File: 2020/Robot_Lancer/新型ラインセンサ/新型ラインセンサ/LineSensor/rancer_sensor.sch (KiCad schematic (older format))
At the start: 31 parts, among them P1 XH_08, U1 S7136, U2 TPR-105F, U3 TPR-105F, U4 S7136, U5 S7136

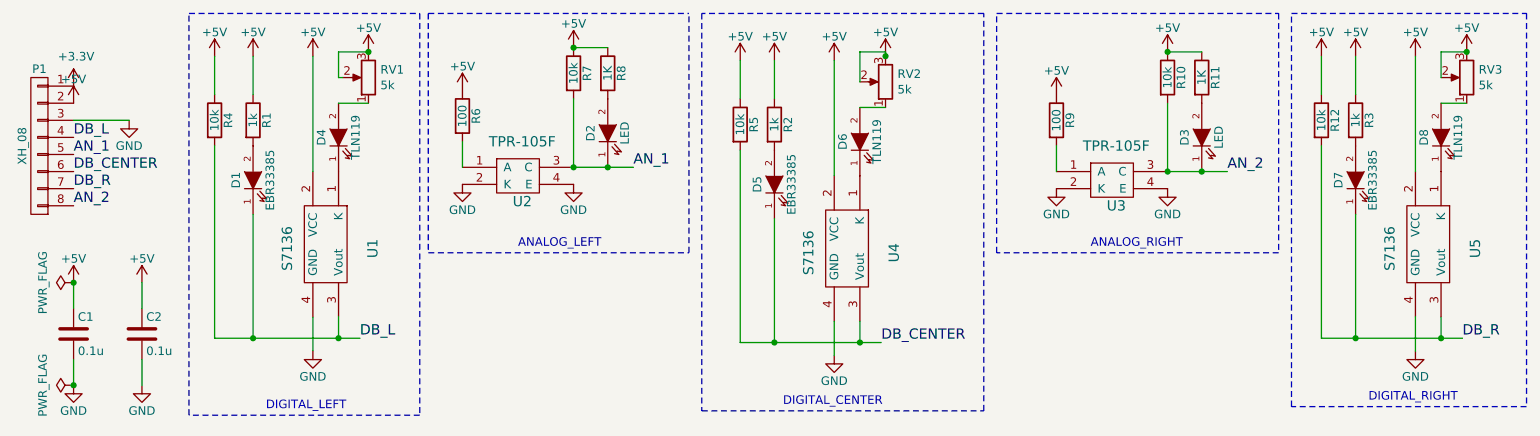
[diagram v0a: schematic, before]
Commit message: 小谷ランサー基板
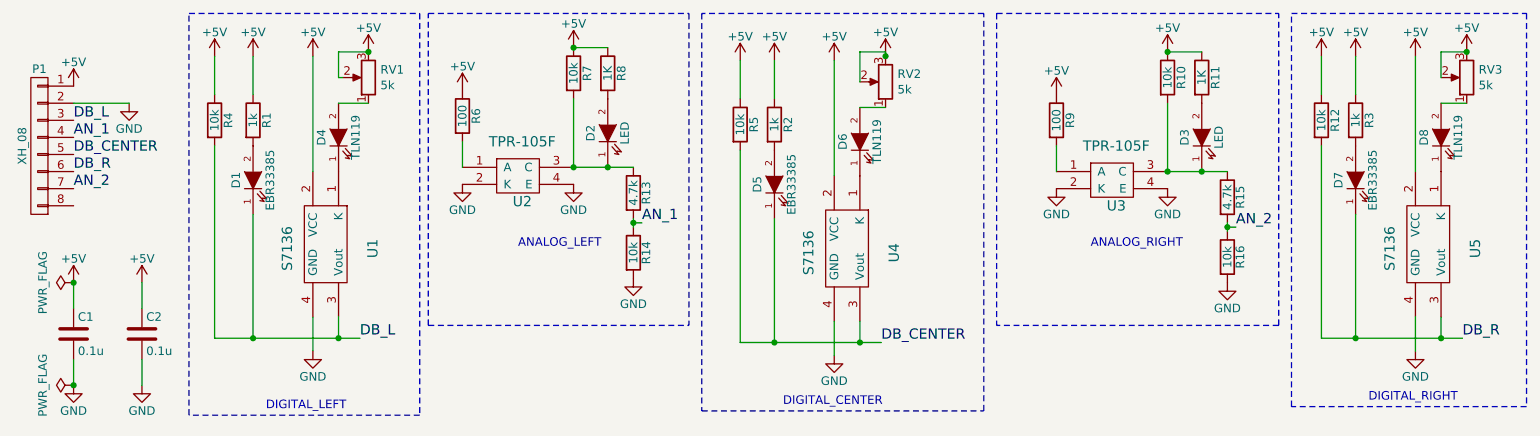
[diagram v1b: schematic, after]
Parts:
- added R13, R15: 4.7k, Mizz_lib:1608_WP, symbol Device:R
- added R14, R16: 10k, Mizz_lib:1608_WP, symbol Device:R
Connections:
- net +3V3 is gone; now on net +5V: P1.1 (P1)
- net +5V: no longer P1.2 (P2)
- net AN_1: now also P1.4 (P4), R13.2, R14.1; no longer D2.1 (K), P1.5 (P5), R7.2, U2.3 (C)
- net AN_2: now also P1.7 (P7), R15.2, R16.1; no longer D3.1 (K), P1.8 (P8), R10.2, U3.3 (C)
- net DB_CENTER: now also P1.5 (P5); no longer P1.6 (P6)
- net DB_L: now also P1.3 (P3); no longer P1.4 (P4)
- net DB_R: now also P1.6 (P6); no longer P1.7 (P7)
- net GND: now also P1.2 (P2), R14.2, R16.2; no longer P1.3 (P3)
- new net: D2.1 (K), R13.1, R7.2, U2.3 (C)
- new net: D3.1 (K), R10.2, R15.1, U3.3 (C)
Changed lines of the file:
@@
 L power:+5V #PWR03
 U 1 1 5C5036D6
-P 1750 3275
-F 0 "#PWR03" H 1750 3125 50  0001 C CNN
-F 1 "+5V" H 1750 3415 50  0000 C CNN
-F 2 "" H 1750 3275 50  0000 C CNN
-F 3 "" H 1750 3275 50  0000 C CNN
-	1    1750 3275
+P 1750 3175
+F 0 "#PWR03" H 1750 3025 50  0001 C CNN
+F 1 "+5V" H 1750 3315 50  0000 C CNN
+F 2 "" H 1750 3175 50  0000 C CNN
+F 3 "" H 1750 3175 50  0000 C CNN
+	1    1750 3175
 	1    0    0    -1
 $EndComp
@@
 L power:GND #PWR04
 U 1 1 5C5036EA
-P 2075 3375
-F 0 "#PWR04" H 2075 3125 50  0001 C CNN
-F 1 "GND" H 2075 3225 50  0000 C CNN
-F 2 "" H 2075 3375 50  0000 C CNN
-F 3 "" H 2075 3375 50  0000 C CNN
-	1    2075 3375
+P 2075 3275
+F 0 "#PWR04" H 2075 3025 50  0001 C CNN
+F 1 "GND" H 2075 3125 50  0000 C CNN
+F 2 "" H 2075 3275 50  0000 C CNN
+F 3 "" H 2075 3275 50  0000 C CNN
+	1    2075 3275
 	1    0    0    -1
 $EndComp
@@
 	-1   0    0    -1
 $EndComp
-Text Label 1750 3575 0    60   ~ 0
+Text Label 1750 3475 0    60   ~ 0
 AN_1
-Text Label 1750 3875 0    60   ~ 0
+Text Label 1750 3775 0    60   ~ 0
 AN_2
 $Comp
@@
 	1    0    0    -1
 $EndComp
-Text Label 5025 3650 0    60   ~ 0
+Text Label 5075 3975 0    60   ~ 0
 AN_1
 Wire Wire Line
@@
 	8150 3675 8350 3675
 Connection ~ 8350 3675
-Text Label 8500 3675 0    60   ~ 0
+Text Label 8550 4000 0    60   ~ 0
 AN_2
 $Comp
@@
 Wire Wire Line
 	9250 3925 9250 4650
-Text Label 1750 3475 0    60   ~ 0
+Text Label 1750 3375 0    60   ~ 0
 DB_L
-Text Label 1750 3775 0    60   ~ 0
+Text Label 1750 3675 0    60   ~ 0
 DB_R
-Text Label 1750 3675 0    60   ~ 0
+Text Label 1750 3575 0    60   ~ 0
 DB_CENTER
 $Comp
@@
 DIGITAL_RIGHT
 Wire Notes Line
-	3825 2750 3825 4150
-Wire Notes Line
-	3825 4150 5350 4150
-Wire Notes Line
-	5350 4150 5350 2750
+	3825 4575 5350 4575
 Wire Notes Line
 	3825 2750 5350 2750
@@
 Connection ~ 4675 3650
 Wire Notes Line
-	8800 2750 8800 4150
-Wire Notes Line
-	8800 4150 7150 4150
-Wire Notes Line
-	7150 4150 7150 2750
+	8800 4575 7150 4575
 Wire Notes Line
 	7150 2750 8800 2750
@@
 Connection ~ 1750 4925
 Wire Wire Line
-	2075 3375 1750 3375
-$Comp
-L power:+3.3V #PWR?
-U 1 1 5E149DB0
-P 1750 3175
-F 0 "#PWR?" H 1750 3025 50  0001 C CNN
-F 1 "+3.3V" H 1765 3348 50  0000 C CNN
-F 2 "" H 1750 3175 50  0001 C CNN
-F 3 "" H 1750 3175 50  0001 C CNN
-	1    1750 3175
-	1    0    0    -1
-$EndComp
+	2075 3275 1750 3275
+$Comp
+L Device:R R15
+U 1 1 5E18896D
+P 8500 3825
+F 0 "R15" V 8575 3825 50  0000 C CNN
+F 1 "4.7k" V 8500 3825 50  0000 C CNN
+F 2 "Mizz_lib:1608_WP" V 8430 3825 50  0001 C CNN
+F 3 "~" H 8500 3825 50  0001 C CNN
+	1    8500 3825
+	1    0    0    -1
+$EndComp
+$Comp
+L Device:R R16
+U 1 1 5E189230
+P 8500 4175
+F 0 "R16" V 8575 4175 50  0000 C CNN
+F 1 "10k" V 8500 4175 50  0000 C CNN
+F 2 "Mizz_lib:1608_WP" V 8430 4175 50  0001 C CNN
+F 3 "~" H 8500 4175 50  0001 C CNN
+	1    8500 4175
+	1    0    0    -1
+$EndComp
+Wire Wire Line
+	8550 4000 8500 4000
+Wire Wire Line
+	8500 4000 8500 3975
+Wire Wire Line
+	8500 4000 8500 4025
+Connection ~ 8500 4000
+$Comp
+L power:GND #PWR0102
+U 1 1 5E18CFC3
+P 8500 4325
+F 0 "#PWR0102" H 8500 4075 50  0001 C CNN
+F 1 "GND" H 8500 4175 50  0000 C CNN
+F 2 "" H 8500 4325 50  0000 C CNN
+F 3 "" H 8500 4325 50  0000 C CNN
+	1    8500 4325
+	1    0    0    -1
+$EndComp
+Wire Notes Line
+	7150 2750 7150 4575
+Wire Notes Line
+	8800 4575 8800 2750
+Wire Notes Line
+	5350 2750 5350 4575
+Wire Notes Line
+	3825 4575 3825 2750
+$Comp
+L Device:R R13
+U 1 1 5E1947A4
+P 5025 3800
+F 0 "R13" V 5100 3800 50  0000 C CNN
+F 1 "4.7k" V 5025 3800 50  0000 C CNN
+F 2 "Mizz_lib:1608_WP" V 4955 3800 50  0001 C CNN
+F 3 "~" H 5025 3800 50  0001 C CNN
+	1    5025 3800
+	1    0    0    -1
+$EndComp
+$Comp
+L Device:R R14
+U 1 1 5E1947AE
+P 5025 4150
+F 0 "R14" V 5100 4150 50  0000 C CNN
+F 1 "10k" V 5025 4150 50  0000 C CNN
+F 2 "Mizz_lib:1608_WP" V 4955 4150 50  0001 C CNN
+F 3 "~" H 5025 4150 50  0001 C CNN
+	1    5025 4150
+	1    0    0    -1
+$EndComp
+Wire Wire Line
+	5075 3975 5025 3975
+Wire Wire Line
+	5025 3975 5025 3950
+Wire Wire Line
+	5025 3975 5025 4000
+Connection ~ 5025 3975
+$Comp
+L power:GND #PWR0103
+U 1 1 5E1947BC
+P 5025 4300
+F 0 "#PWR0103" H 5025 4050 50  0001 C CNN
+F 1 "GND" H 5025 4150 50  0000 C CNN
+F 2 "" H 5025 4300 50  0000 C CNN
+F 3 "" H 5025 4300 50  0000 C CNN
+	1    5025 4300
+	1    0    0    -1
+$EndComp
